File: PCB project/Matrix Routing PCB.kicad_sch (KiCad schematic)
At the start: 14 parts, among them J1 53261-0471, J2 JST_PH_S4B-PH-SM4-TB, J3 ESQ-105-12-T-D, J4 TSM-102-01-L-DH-A, J5 USB-A-S-F-B-SM2-R-TR, U1 FT232RL

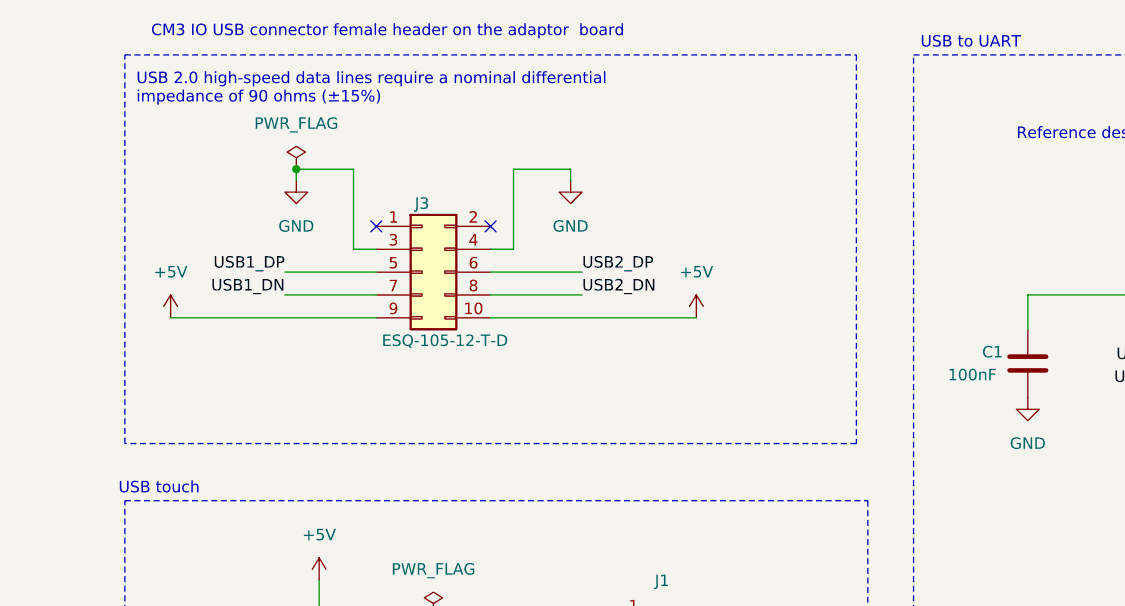
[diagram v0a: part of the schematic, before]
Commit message: Commit after review
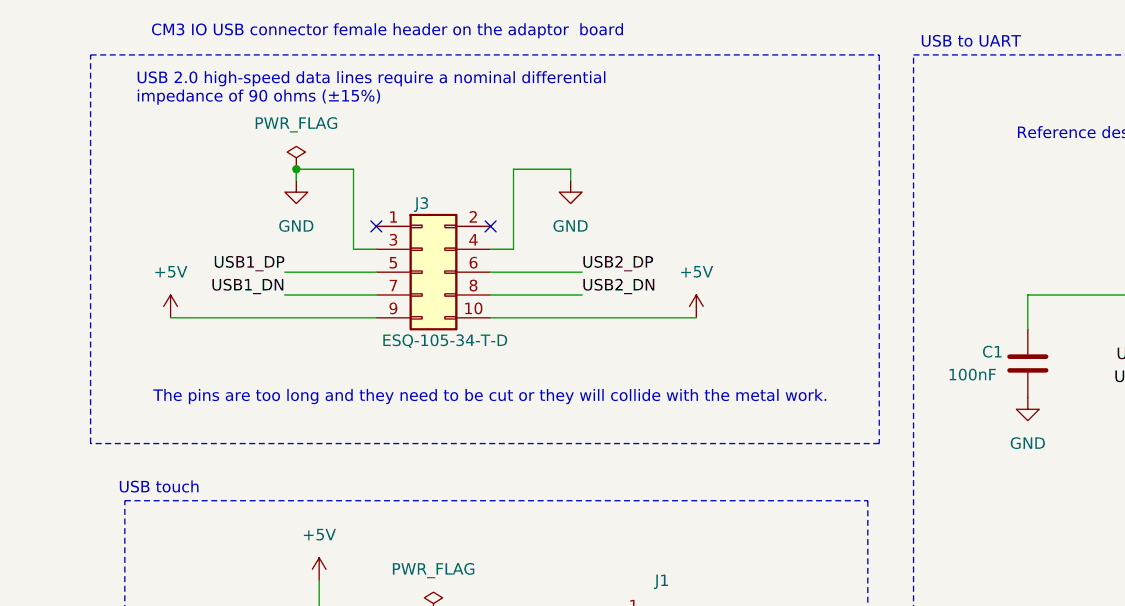
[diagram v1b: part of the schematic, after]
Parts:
- J3: value ESQ-105-12-T-D -> ESQ-105-34-T-D; Digikey PN SAM15563-ND -> ESQ-105-33-T-D-ND; MPN ESQ-105-12-T-D -> ESQ-105-33-T-D; RS PN 208-1157 -> 208-1163
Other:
- note added: "The pins are too long and they need to be cut or they will collide with the metal work."
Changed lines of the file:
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@@
 	)
 	(rectangle
-		(start 77.47 46.99)
-		(end 158.75 90.17)
+		(start 73.66 46.99)
+		(end 161.29 90.17)
 		(stroke
 			(width 0)
@@
 		(exclude_from_sim no)
 		(at 171.45 45.72 0)
+		(effects
+			(font
+				(size 1.27 1.27)
+			)
+		)
+	)
+	(text "The pins are too long and they need to be cut or they will collide with the metal work."
+		(exclude_from_sim no)
+		(at 118.11 85.09 0)
 		(effects
 			(font
@@
 			)
 		)
-		(property "Value" "ESQ-105-12-T-D"
+		(property "Value" "ESQ-105-34-T-D"
 			(at 113.03 78.74 0)
 			(show_name no)
@@
 			)
 		)
-		(property "Digikey PN" "SAM15563-ND"
+		(property "Digikey PN" "ESQ-105-33-T-D-ND"
 			(at 110.49 71.12 0)
 			(hide yes)
@@
 			)
 		)
-		(property "MPN" "ESQ-105-12-T-D"
+		(property "MPN" "ESQ-105-33-T-D"
 			(at 110.49 71.12 0)
 			(hide yes)
@@
 			)
 		)
-		(property "RS PN" " 208-1157"
+		(property "RS PN" "208-1163"
 			(at 110.49 71.12 0)
 			(hide yes)
